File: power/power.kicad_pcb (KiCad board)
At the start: 2 copper layers, 108.2 x 81.5 mm, 2 parts, among them J1 ET60T-D04-3-08-D04-X-R1-S, J2 796636-6

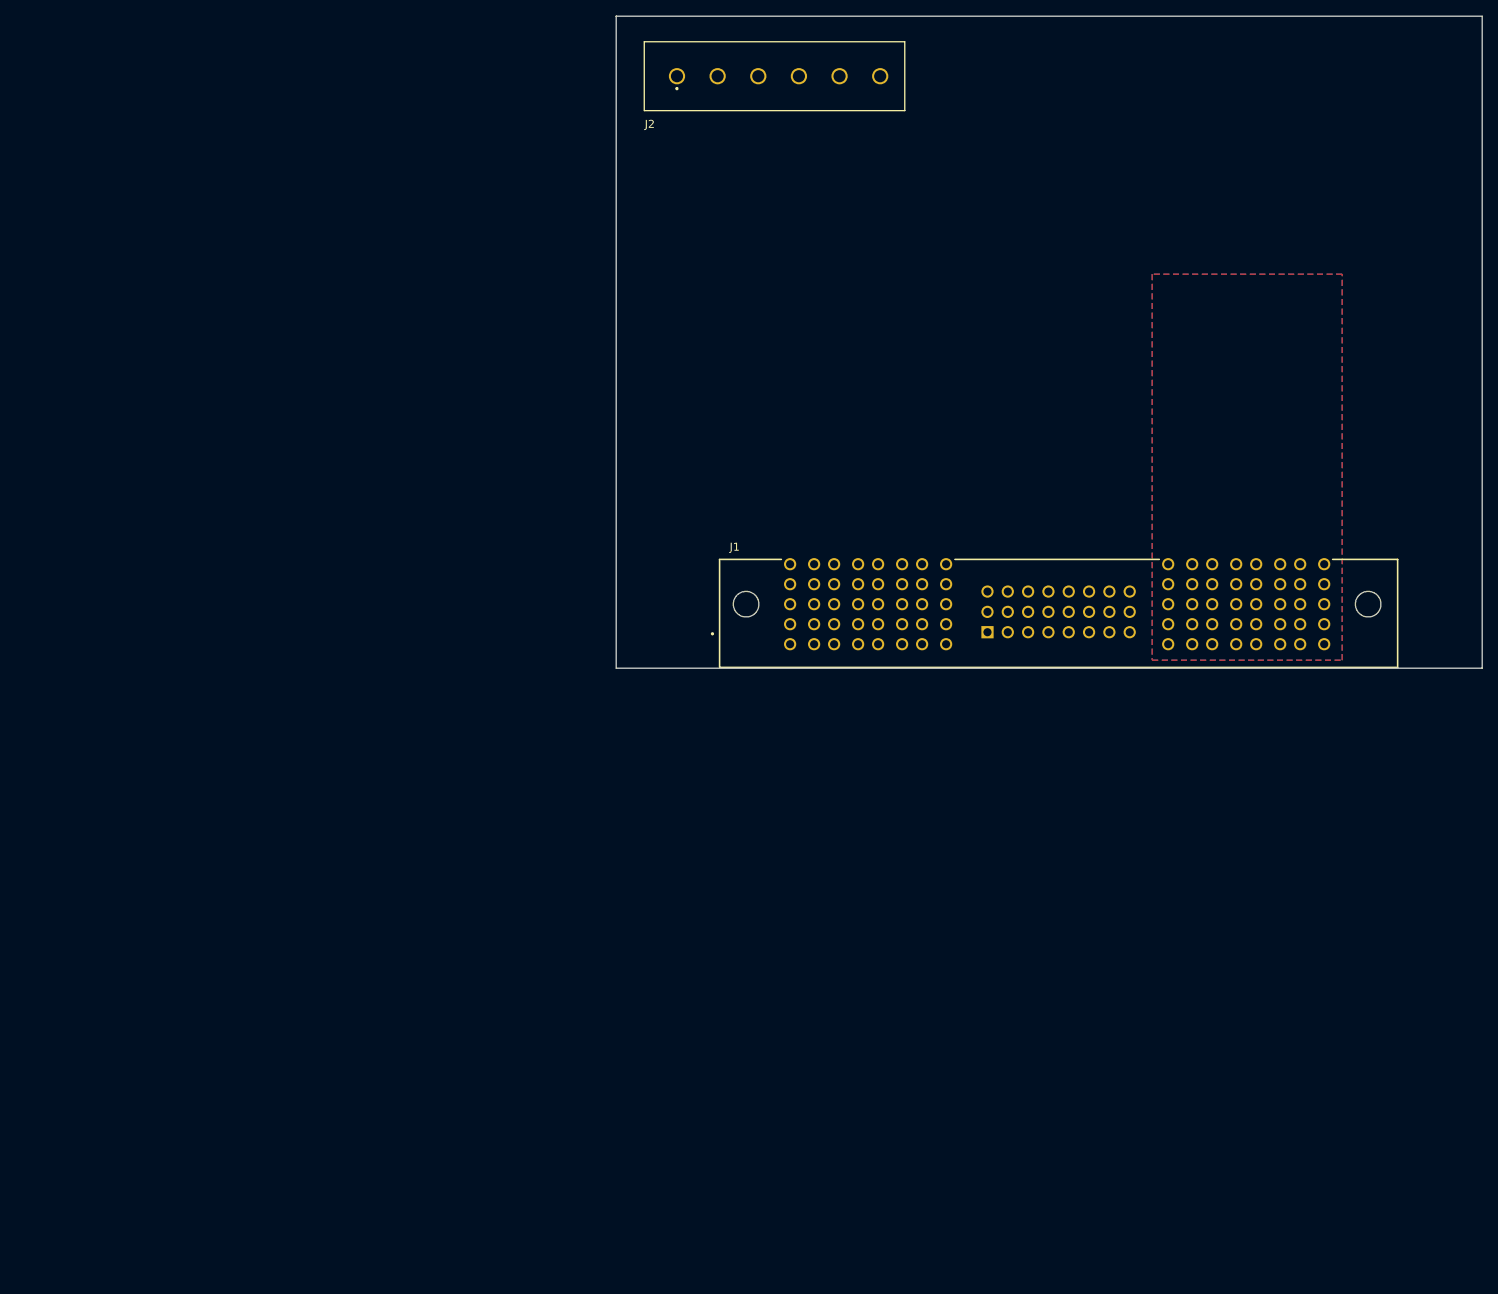
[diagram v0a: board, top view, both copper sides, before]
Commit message: work
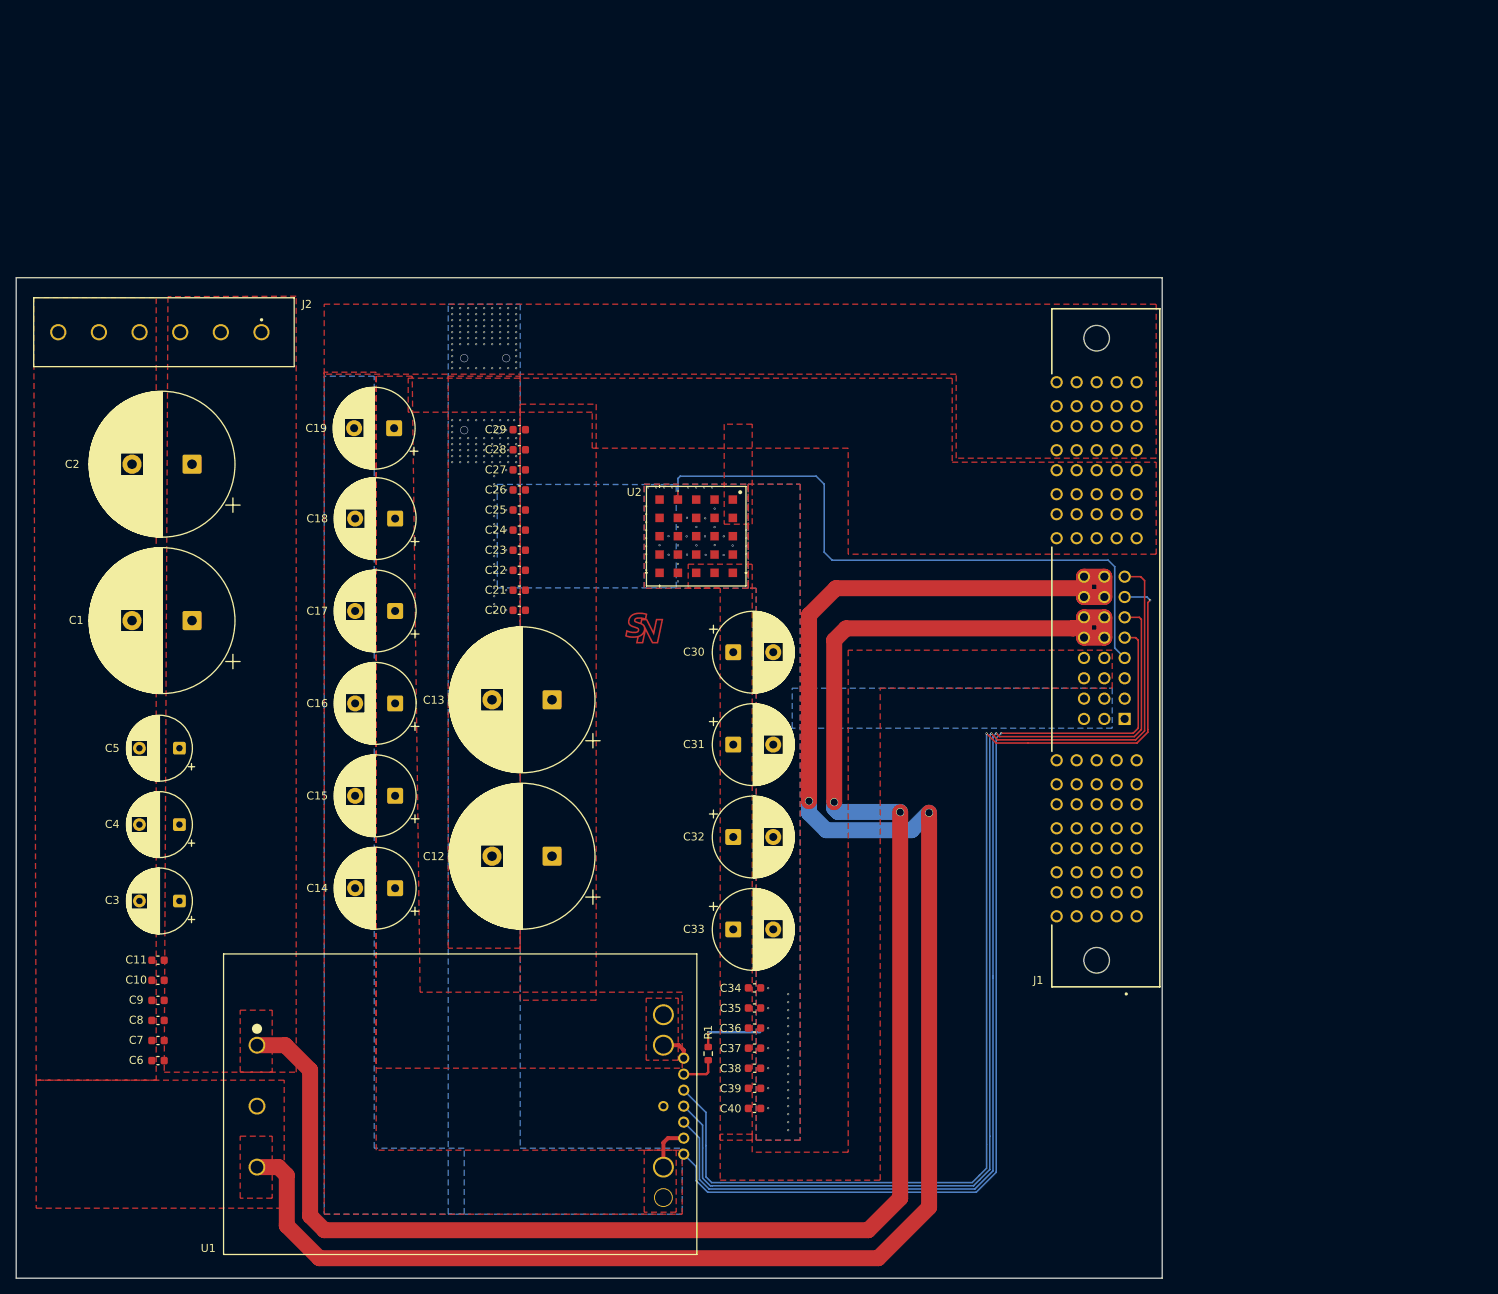
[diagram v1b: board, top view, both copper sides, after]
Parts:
- added C1: C_Polarized_Small, Capacitor_THT:CP_Radial_D18.0mm_P7.50mm, F.Cu at (47.5, 102.5)
- added C10: C_Small, Capacitor_SMD:C_0603_1608Metric, F.Cu at (43.2, 147.5)
- added C11: C_Small, Capacitor_SMD:C_0603_1608Metric, F.Cu at (43.2, 145.0)
- added C12: C_Polarized_Small, Capacitor_THT:CP_Radial_D18.0mm_P7.50mm, F.Cu at (92.5, 132.0)
- added C13: C_Polarized_Small, Capacitor_THT:CP_Radial_D18.0mm_P7.50mm, F.Cu at (92.5, 112.5)
- added C14: C_Polarized_Small, Capacitor_THT:CP_Radial_D10.0mm_P5.00mm, F.Cu at (72.9, 136.0)
- added C15: C_Polarized_Small, Capacitor_THT:CP_Radial_D10.0mm_P5.00mm, F.Cu at (72.9, 124.5)
- added C16: C_Polarized_Small, Capacitor_THT:CP_Radial_D10.0mm_P5.00mm, F.Cu at (72.9, 112.9)
- added C17: C_Polarized_Small, Capacitor_THT:CP_Radial_D10.0mm_P5.00mm, F.Cu at (72.9, 101.3)
- added C18: C_Polarized_Small, Capacitor_THT:CP_Radial_D10.0mm_P5.00mm, F.Cu at (72.9, 89.8)
- added C19: C_Polarized_Small, Capacitor_THT:CP_Radial_D10.0mm_P5.00mm, F.Cu at (72.7, 78.5)
- added C2: C_Polarized_Small, Capacitor_THT:CP_Radial_D18.0mm_P7.50mm, F.Cu at (47.5, 83.0)
- added C20: C_Small, Capacitor_SMD:C_0603_1608Metric, F.Cu at (88.4, 101.3)
- added C21: C_Small, Capacitor_SMD:C_0603_1608Metric, F.Cu at (88.4, 98.8)
- added C22: C_Small, Capacitor_SMD:C_0603_1608Metric, F.Cu at (88.4, 96.3)
- added C23: C_Small, Capacitor_SMD:C_0603_1608Metric, F.Cu at (88.4, 93.8)
- added C24: C_Small, Capacitor_SMD:C_0603_1608Metric, F.Cu at (88.4, 91.2)
- added C25: C_Small, Capacitor_SMD:C_0603_1608Metric, F.Cu at (88.4, 88.7)
- added C26: C_Small, Capacitor_SMD:C_0603_1608Metric, F.Cu at (88.4, 86.2)
- added C27: C_Small, Capacitor_SMD:C_0603_1608Metric, F.Cu at (88.4, 83.7)
- added C28: C_Small, Capacitor_SMD:C_0603_1608Metric, F.Cu at (88.4, 81.2)
- added C29: C_Small, Capacitor_SMD:C_0603_1608Metric, F.Cu at (88.4, 78.7)
- added C3: C_Polarized_Small, Capacitor_THT:CP_Radial_D8.0mm_P5.00mm, F.Cu at (45.9, 137.6)
- added C30: C_Polarized_Small, Capacitor_THT:CP_Radial_D10.0mm_P5.00mm, F.Cu at (115.1, 106.5)
- added C31: C_Polarized_Small, Capacitor_THT:CP_Radial_D10.0mm_P5.00mm, F.Cu at (115.1, 118.0)
- added C32: C_Polarized_Small, Capacitor_THT:CP_Radial_D10.0mm_P5.00mm, F.Cu at (115.1, 129.6)
- added C33: C_Polarized_Small, Capacitor_THT:CP_Radial_D10.0mm_P5.00mm, F.Cu at (115.1, 141.2)
- added C34: C_Small, Capacitor_SMD:C_0603_1608Metric, F.Cu at (117.8, 148.5)
- added C35: C_Small, Capacitor_SMD:C_0603_1608Metric, F.Cu at (117.8, 151.0)
- added C36: C_Small, Capacitor_SMD:C_0603_1608Metric, F.Cu at (117.8, 153.5)
- added C37: C_Small, Capacitor_SMD:C_0603_1608Metric, F.Cu at (117.8, 156.0)
- added C38: C_Small, Capacitor_SMD:C_0603_1608Metric, F.Cu at (117.8, 158.5)
- added C39: C_Small, Capacitor_SMD:C_0603_1608Metric, F.Cu at (117.8, 161.0)
- added C4: C_Polarized_Small, Capacitor_THT:CP_Radial_D8.0mm_P5.00mm, F.Cu at (45.9, 128.1)
- added C40: C_Small, Capacitor_SMD:C_0603_1608Metric, F.Cu at (117.8, 163.5)
- added C5: C_Polarized_Small, Capacitor_THT:CP_Radial_D8.0mm_P5.00mm, F.Cu at (45.9, 118.5)
- added C6: C_Small, Capacitor_SMD:C_0603_1608Metric, F.Cu at (43.2, 157.6)
- added C7: C_Small, Capacitor_SMD:C_0603_1608Metric, F.Cu at (43.2, 155.0)
- added C8: C_Small, Capacitor_SMD:C_0603_1608Metric, F.Cu at (43.2, 152.5)
- added C9: C_Small, Capacitor_SMD:C_0603_1608Metric, F.Cu at (43.2, 150.0)
- added G1: LOGO, custom:logo, F.Cu at (104.0, 103.5)
- added R1: 10k, Resistor_SMD:R_0603_1608Metric, F.Cu at (112.0, 156.7)
- added U1: BMR4912510/871, power_symbols:BMR491_FPM, F.Cu at (55.6, 155.6)
- added U2: RPM5.0-6.0, power_symbols:RPM5.0-6.0, F.Cu at (110.5, 92.0)
- moved J2 61.0 mm to (56.2, 66.5), turned to 180 degrees
- moved J1 7.49 mm to (160.6, 106.1), turned to 90 degrees
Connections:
- J1 pad 04: unconnected-(J1-Pad04) -> /RPM_PG
- J1 pad 05: unconnected-(J1-Pad05) -> /BMR_PG
- J1 pad 06: unconnected-(J1-Pad06) -> /BMR_SDA
- J1 pad 07: unconnected-(J1-Pad07) -> /BMR_SCL
- J1 pad 08: unconnected-(J1-Pad08) -> /BMR_SALERT
- J1 pad 09: 5V_GND -> 12V_GND
- J1 pad 10: 5V_GND -> 12V_GND
- J1 pad 17: 5V_GND -> 12V_GND
- J1 pad 18: 5V_GND -> 12V_GND
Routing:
- net 48V_GND: track 0.00 -> 233.3 mm, vias 0 -> 2
- net +48V: track 0.00 -> 222.0 mm, vias 0 -> 2
- net /BMR_SCL: track 0.00 -> 143.6 mm, vias 0 -> 2
- net /BMR_SALERT: track 0.00 -> 143.1 mm, vias 0 -> 1
- net /BMR_SDA: track 0.00 -> 135.9 mm, vias 0 -> 1
- net /BMR_PG: track 0.00 -> 128.4 mm, vias 0 -> 1
- net /RPM_PG: track 0.00 -> 78.9 mm, vias 0 -> 1
- net 12V_GND: track 0.00 -> 14.2 mm, vias 0 -> 232
- net Net-(U1-SA1): track 0.00 -> 4.66 mm
- net +12V: track 0.00 -> 3.80 mm
- added copper zone on F.Cu, net +48V
- added copper zone on F.Cu, net +5V
- added copper zone on F.Cu, net 12V_GND
- added copper zone on F.Cu, net 48V_GND
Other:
- board size 108.2 x 81.5 mm -> 143.2 x 125.1 mm

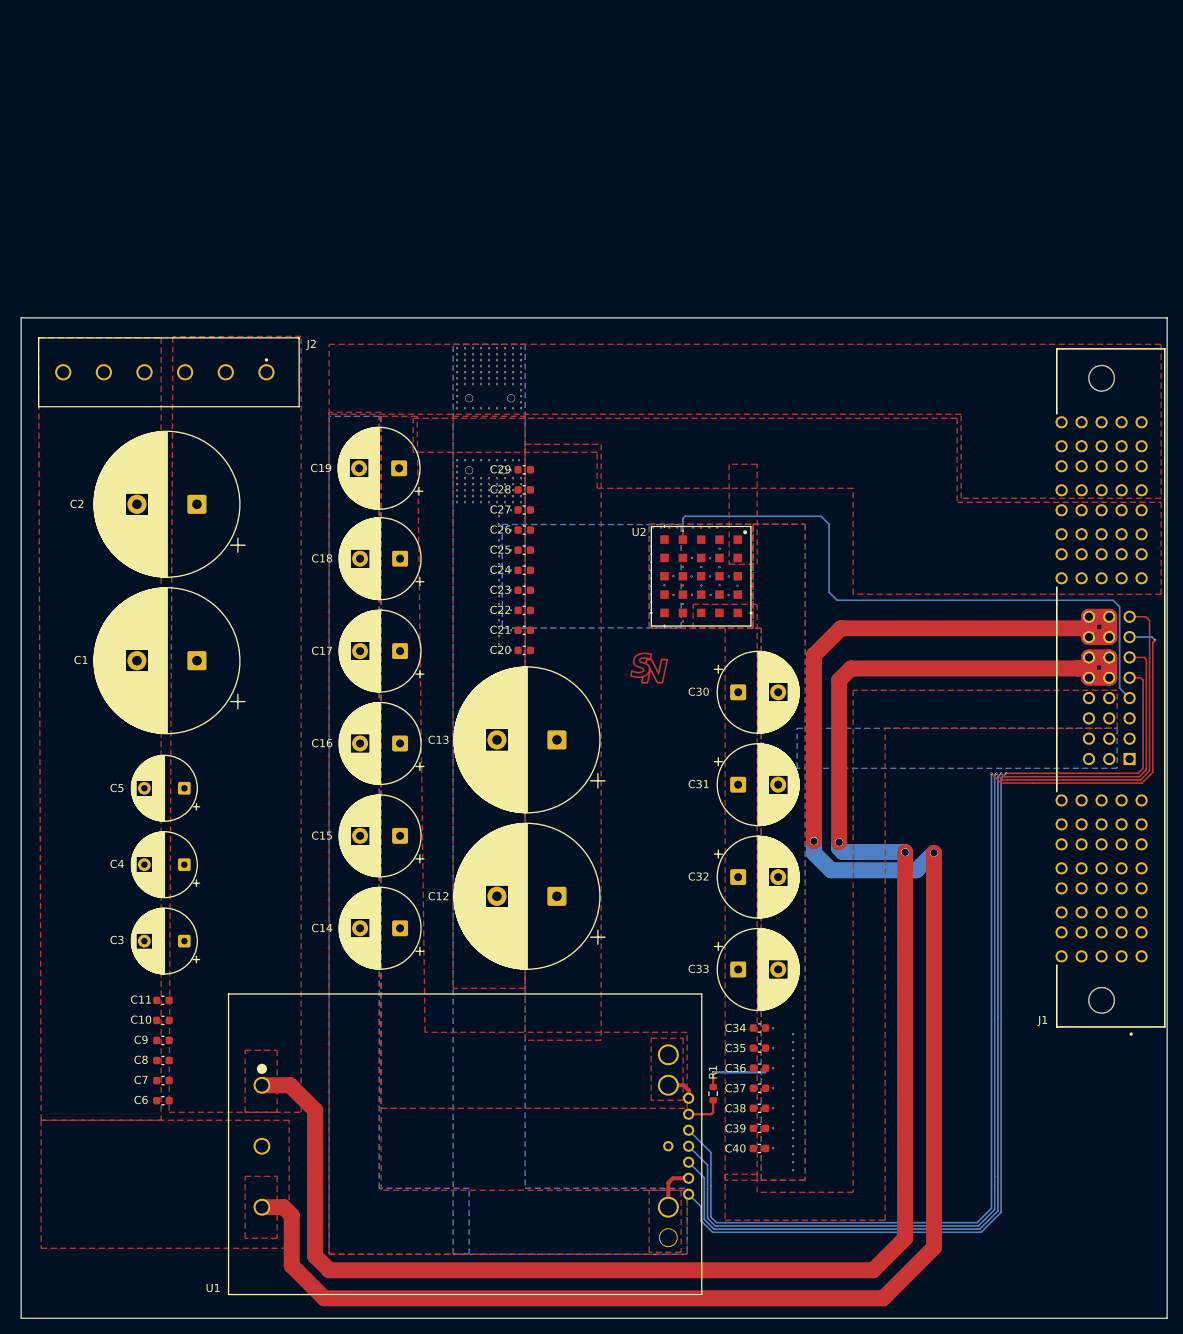
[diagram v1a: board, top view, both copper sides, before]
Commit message: stuff
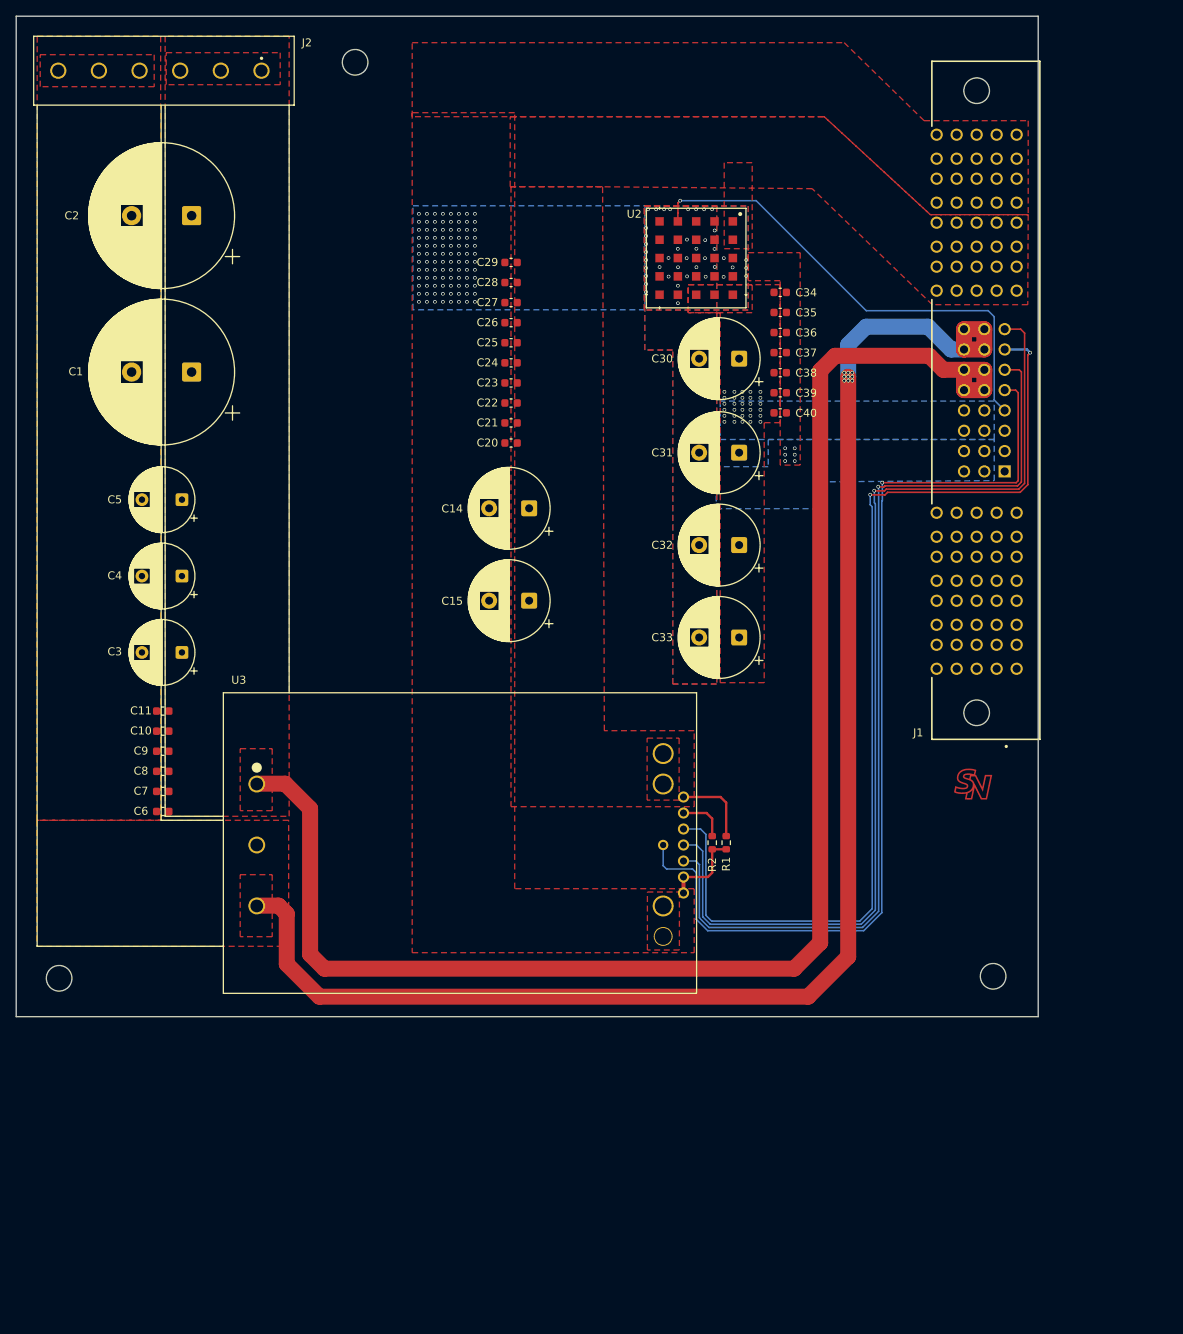
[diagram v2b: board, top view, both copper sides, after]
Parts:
- removed C12, C13: C_Polarized_Small, Capacitor_THT:CP_Radial_D18.0mm_P7.50mm
- removed C16, C17, C18, C19: C_Polarized_Small, Capacitor_THT:CP_Radial_D10.0mm_P5.00mm
- removed U1: BMR4912510/871, power_symbols:BMR491_FPM
- added H1: MountingHole, MountingHole:MountingHole_3.2mm_M3, F.Cu at (30.2, 142.2)
- added H2: MountingHole, MountingHole:MountingHole_3.2mm_M3, F.Cu at (67.2, 27.8)
- added H3: MountingHole, MountingHole:MountingHole_3.2mm_M3, F.Cu at (147.0, 142.0)
- added R2: 10k, Resistor_SMD:R_0603_1608Metric, F.Cu at (111.9, 125.3)
- added U3: BMR4800116/005, power_symbols:BMR491_FPM, F.Cu at (55.0, 118.0)
- moved C38 92.0 mm to (120.4, 66.5)
- moved C34 92.0 mm to (120.4, 56.5)
- moved C35 92.0 mm to (120.4, 59.0)
- moved C36 92.0 mm to (120.4, 61.5)
- moved C39 92.0 mm to (120.4, 69.1)
- moved C40 92.0 mm to (120.4, 71.6)
- moved C37 92.0 mm to (120.4, 64.0)
- moved C14 54.9 mm to (89.0, 83.5)
- moved G1 43.0 mm to (144.5, 118.0)
- moved C30 41.7 mm to (115.2, 64.8), turned to 180 degrees
- moved C31 41.5 mm to (115.2, 76.5), turned to 180 degrees
- moved C32 41.5 mm to (115.2, 88.1), turned to 180 degrees
- moved C33 41.5 mm to (115.2, 99.7), turned to 180 degrees
- moved U2 39.8 mm to (109.9, 52.2)
- moved J1 39.2 mm to (144.9, 70.2)
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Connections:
- J1 pad 05: /BMR_PG -> /~{BMR_PG}
- J1 pad 08: /BMR_SALERT -> /~{BMR_SALERT}
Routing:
- net /BMR_SALERT: track 143.1 -> 0.00 mm, vias 1 -> 0
- net /BMR_PG: track 128.4 -> 0.00 mm, vias 1 -> 0
- net /~{BMR_SALERT}: track 0.00 -> 126.8 mm, vias 0 -> 1
- net /~{BMR_PG}: track 0.00 -> 121.3 mm, vias 0 -> 1
- net 48V_GND: track 233.3 -> 189.0 mm, vias 2 -> 9
- net +48V: track 222.0 -> 193.1 mm, vias 2 -> 0
- net /RPM_PG: track 78.9 -> 60.2 mm
- net /BMR_SCL: track 143.6 -> 127.1 mm
- net /BMR_SDA: track 135.9 -> 119.9 mm
- net Net-(U3-SA1): track 0.00 -> 6.06 mm
- net Net-(U3-SA0): track 4.66 -> 9.81 mm
- net +12V: track 3.80 -> 0.00 mm
- net 12V_GND: track 14.2 -> 10.5 mm, vias 232 -> 143
- net +5V: vias 0 -> 30
- added copper zone on B.Cu, net +5V
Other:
- board size 143.2 x 125.1 mm -> 127.8 x 125.1 mm
